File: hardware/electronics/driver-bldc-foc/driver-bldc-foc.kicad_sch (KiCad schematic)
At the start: 23 parts, among them J3 USB_A, J4 Motor_Phase_A, J5 Motor_Phase_B, J6 Motor_Phase_C, J8 XT30PW-M, U1 TPS563240DDC, U3 AP1117-33, U5 TJA1051T-3

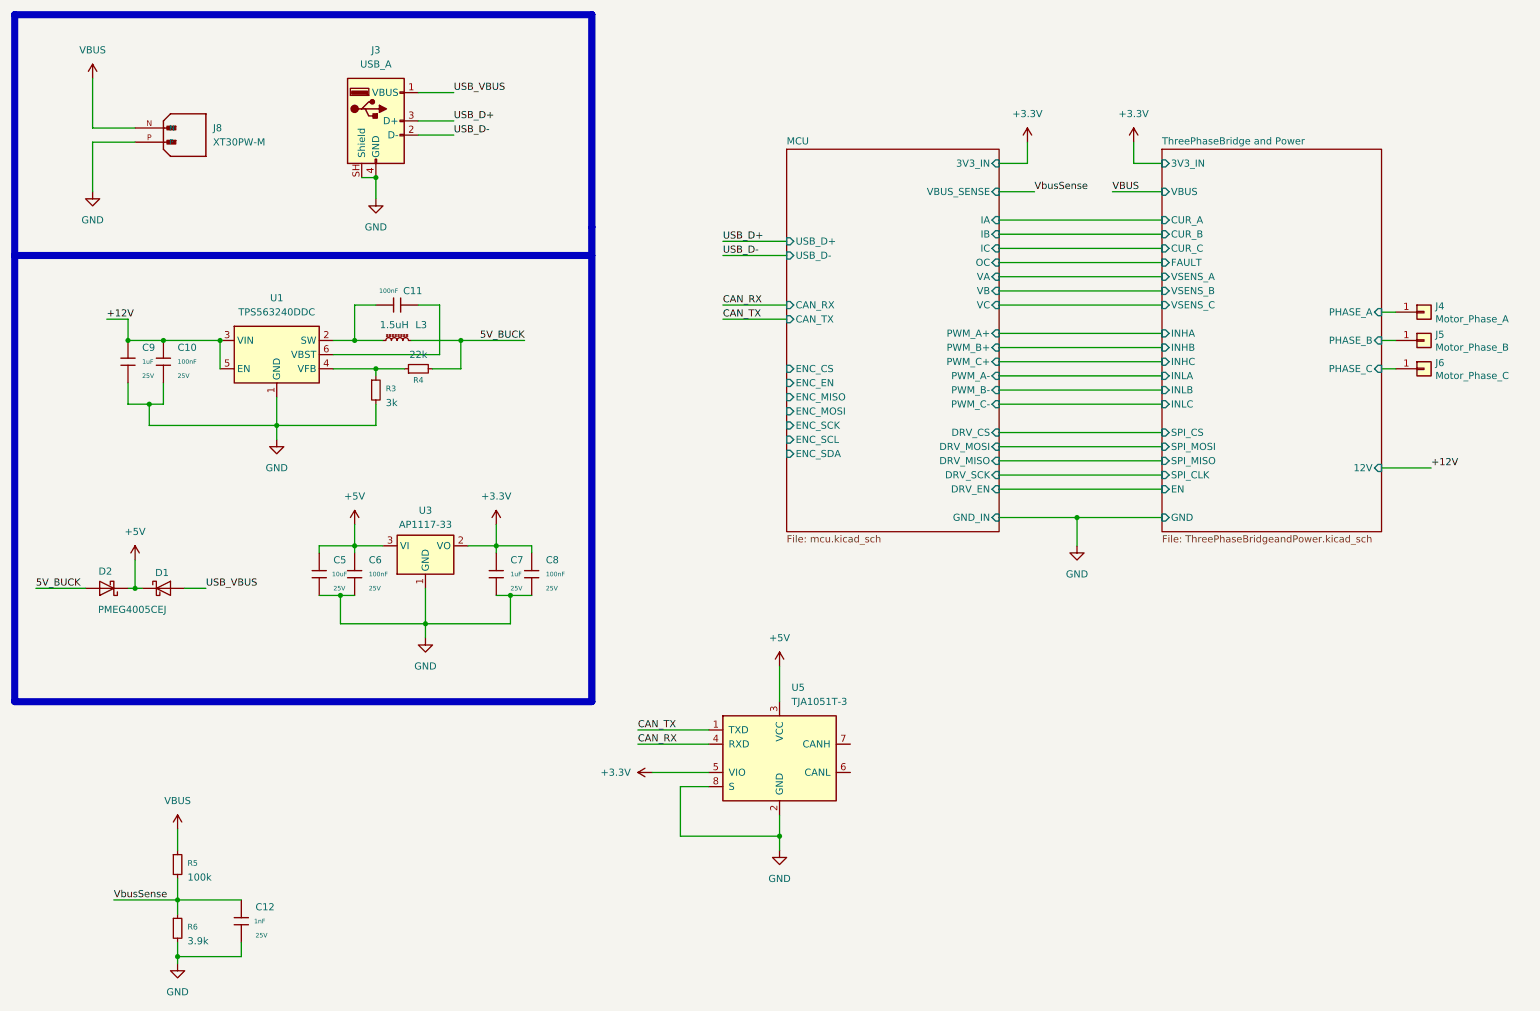
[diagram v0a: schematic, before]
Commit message: update root schematic
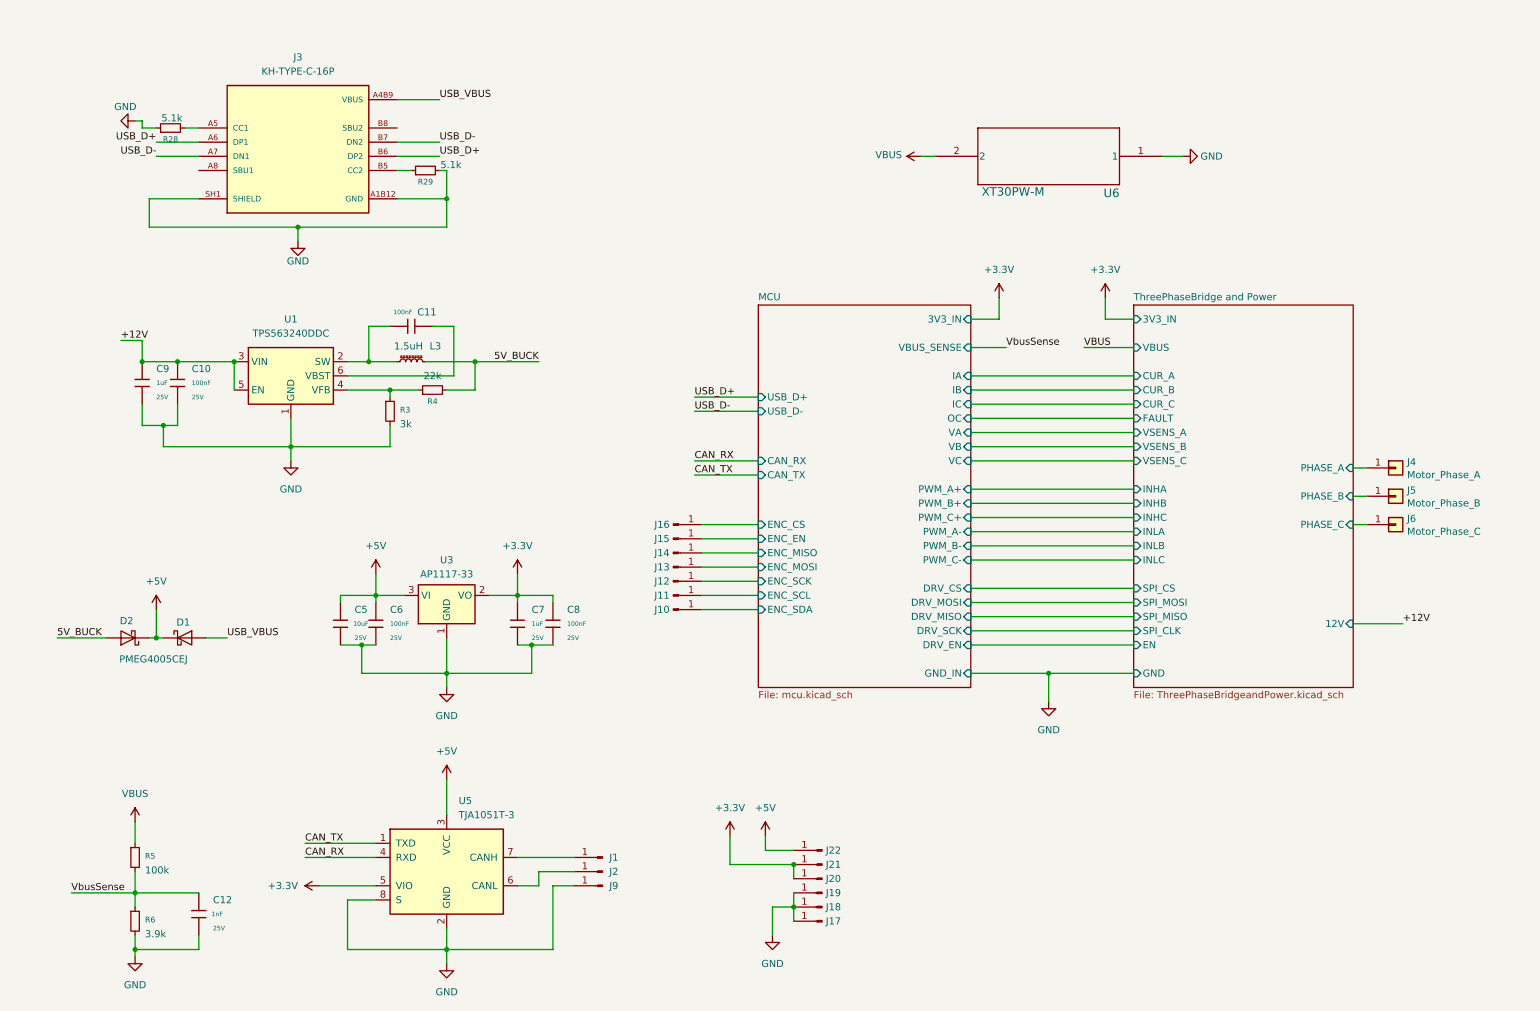
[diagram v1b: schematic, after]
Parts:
- removed J3: USB_A, Connector_USB:USB_B_OST_USB-B1HSxx_Horizontal, symbol Connector:USB_A
- removed J8: XT30PW-M, XT30PW-M:AMASS_XT30PW-M, symbol XT30PW-M:XT30PW-M
- added J1, J10, J11, J12, J13, J14, J15, J16, J17, J18, J19, J2, J20, J21, J22, J9: Conn_01x01_Pin, Connector_Wire:SolderWirePad_1x01_SMD_2x4mm, symbol Connector:Conn_01x01_Pin
- added J3: KH-TYPE-C-16P, KH-TYPE-C-16P:KINGHELM_KH-TYPE-C-16P, symbol KH-TYPE-C-16P:KH-TYPE-C-16P
- added R28, R29: 5.1k, Resistor_SMD:R_0805_2012Metric, symbol Device:R_Small
- added U6: XT30PW-M, XT30PW-M_AMA, symbol 2026-07-22_03-26-08:XT30PW-M
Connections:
- net USB_VBUS is gone; now on net VBUS: D1.2 (A)
- net +3.3V: now also J20.1 (Pin_1), J21.1 (Pin_1)
- net +5V: now also J22.1 (Pin_1)
- net GND: now also J17.1 (Pin_1), J18.1 (Pin_1), J19.1 (Pin_1), J3.A12B1 (GND), J3.A1B12 (GND), J3.SH1 (SHIELD), J3.SH2 (SHIELD), J3.SH3 (SHIELD), J3.SH4 (SHIELD), J9.1 (Pin_1), R28.1, R29.2, U6.1
- net MCU/ENC_CS: now also J16.1 (Pin_1)
- net MCU/ENC_EN: now also J15.1 (Pin_1)
- net MCU/ENC_MISO: now also J14.1 (Pin_1)
- net MCU/ENC_MOSI: now also J13.1 (Pin_1)
- net MCU/ENC_SCK: now also J12.1 (Pin_1)
- net MCU/ENC_SCL: now also J11.1 (Pin_1)
- net MCU/ENC_SDA: now also J10.1 (Pin_1)
- net USB_D+: now also J3.A6 (DP1), J3.B6 (DP2)
- net USB_D-: now also J3.A7 (DN1), J3.B7 (DN2)
- net VBUS: now also J3.A4B9 (VBUS), J3.A9B4 (VBUS), U6.2
- net at U5.6 (CANL): now also J2.1 (Pin_1)
- net at U5.7 (CANH): now also J1.1 (Pin_1)
- new net: J3.A5 (CC1), R28.2
- new net: J3.B5 (CC2), R29.1
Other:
- moved on the sheet: C10, C11, C12, C5, C6, C7, C8, C9, D1, D2, J4, J5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
